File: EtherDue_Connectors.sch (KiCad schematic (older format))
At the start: 14 parts, among them P401 USB_5PIN_SHELL

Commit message: exported cmp-file from PCB and back imported it into the schematic. then exported BOM with kicad2csvbom tool
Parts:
- C401: footprint SMD_Packages:SMD-0402_c -> SM0402
- F401: footprint SMD_Packages:SMD-1812 -> SM1812
- R403: footprint SMD_Packages:SMD-0402_r -> SM0402_r
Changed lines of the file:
@@
 F 0 "R403" V 7830 3800 50  0000 C CNN
 F 1 "10K" V 7750 3800 50  0000 C CNN
-F 2 "SMD_Packages:SMD-0402_r" H 7750 3800 60  0001 C CNN
+F 2 "SM0402_r" H 7750 3800 60  0001 C CNN
 F 3 "" H 7750 3800 60  0001 C CNN
 	1    7750 3800
@@
 F 0 "F401" H 6800 3600 40  0000 C CNN
 F 1 "500mA PTC 1812" H 6700 3700 40  0000 C CNN
-F 2 "SMD_Packages:SMD-1812" H 6700 3550 60  0001 C CNN
+F 2 "SM1812" H 6700 3550 60  0001 C CNN
 F 3 "" H 6700 3550 60  0001 C CNN
 	1    6700 3550
@@
 F 0 "C401" H 6050 3850 50  0000 L CNN
 F 1 "10nF" H 6050 3650 50  0000 L CNN
-F 2 "SMD_Packages:SMD-0402_c" H 6000 3750 60  0001 C CNN
+F 2 "SM0402" H 6000 3750 60  0001 C CNN
 F 3 "" H 6000 3750 60  0001 C CNN
 	1    6000 3750

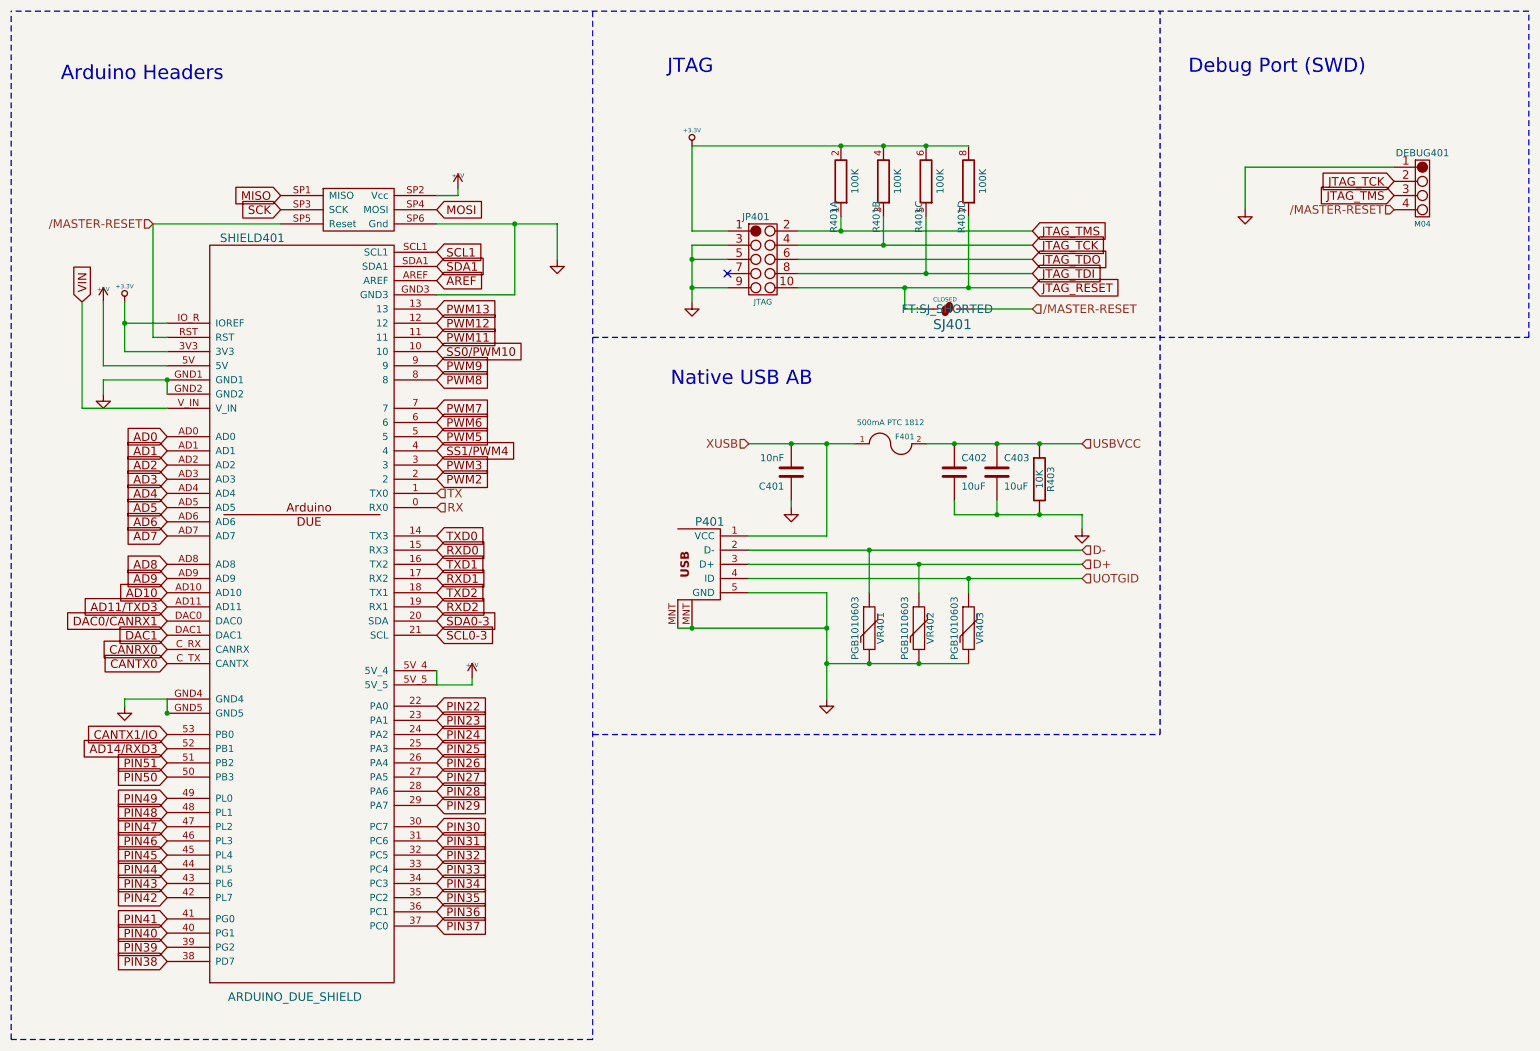
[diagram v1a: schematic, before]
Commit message: Updates im Zuge des Tutorials
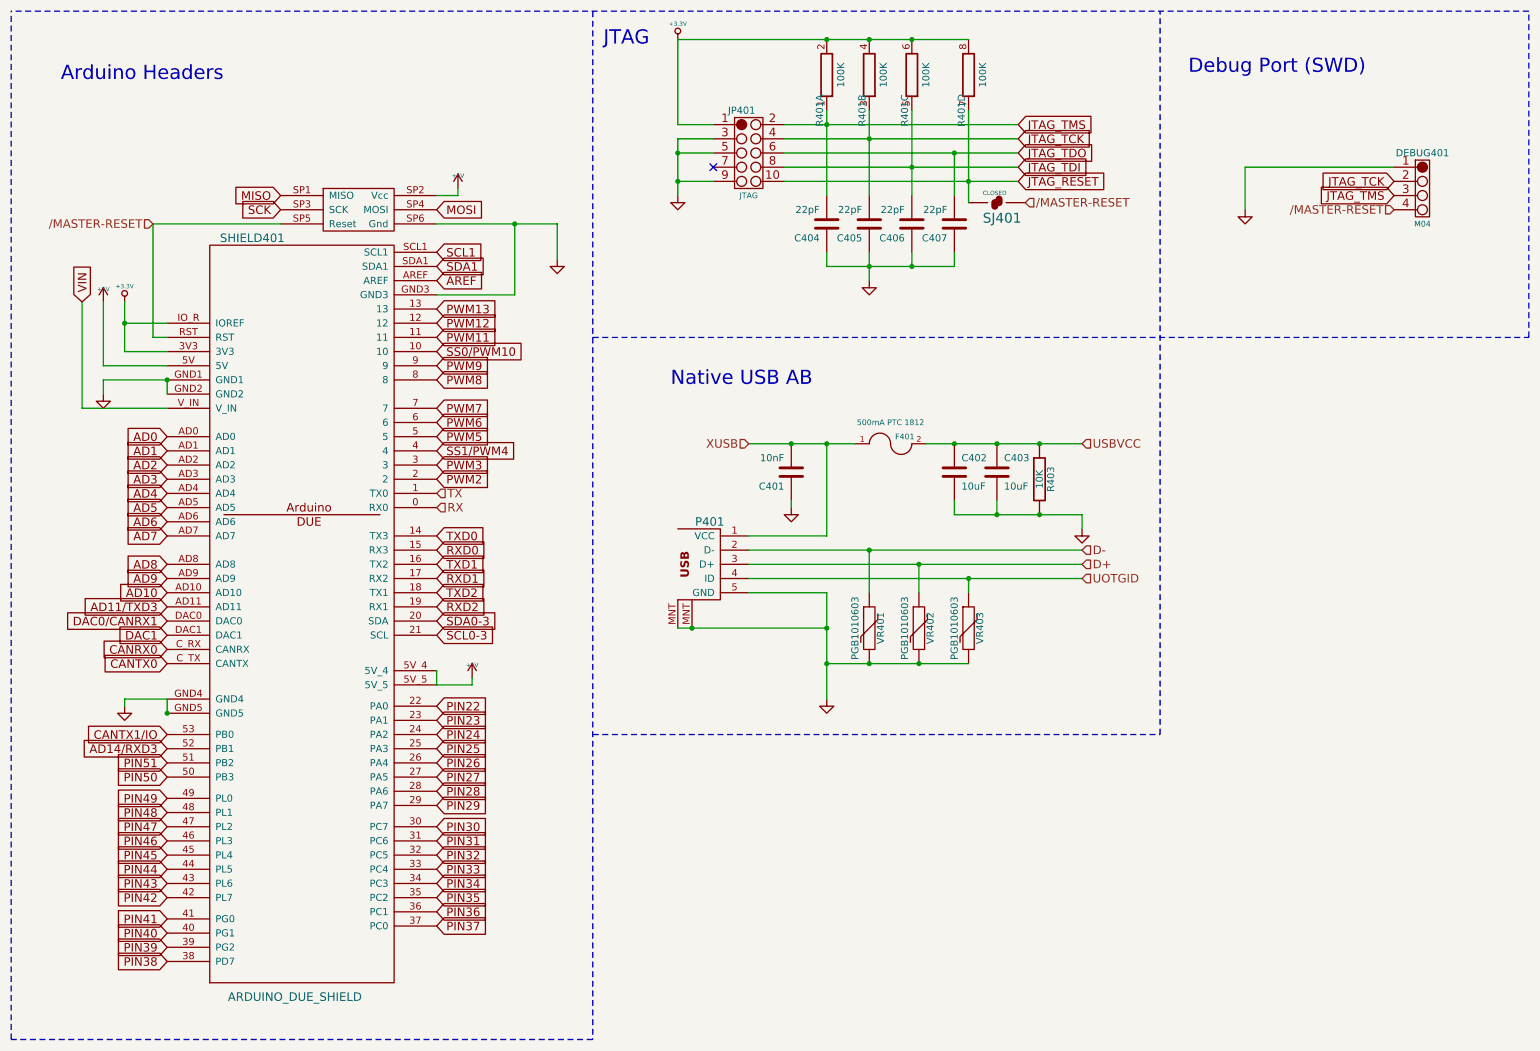
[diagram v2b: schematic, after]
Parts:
- added C404, C405, C406, C407: 22pF, FT:C0402, symbol C
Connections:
- net GND: now also C404.1, C405.1, C406.1, C407.1
- net JTAG_TCK: now also C405.2
- net JTAG_TDI: now also C406.2
- net JTAG_TDO: now also C407.2
- net JTAG_TMS: now also C404.2
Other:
- moved on the sheet: JP401, R401A, R401B, R401C, R401D, SJ401
